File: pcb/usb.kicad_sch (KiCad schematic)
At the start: 16 parts, among them J601 USB_AB_Micro, J602 USB_B_Micro, J604 USB_B_Micro, U601 USBLC6-2P6, U602 CP2102N-Axx-xQFN20, U605 USBLC6-2P6

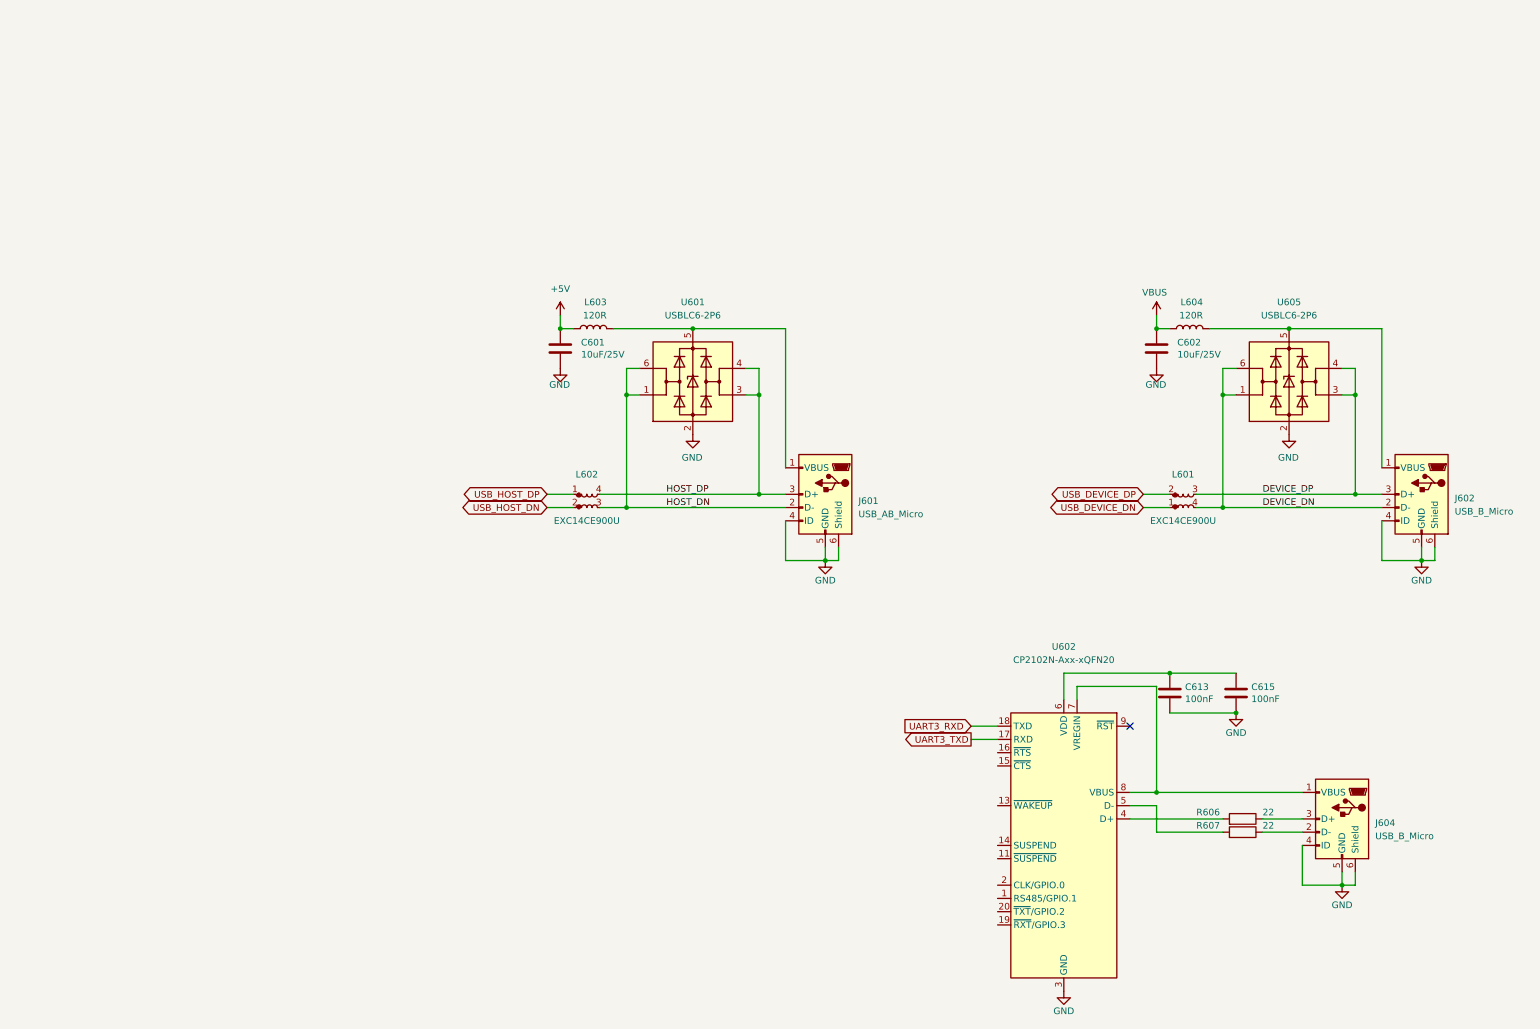
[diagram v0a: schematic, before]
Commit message: pcb: getting ready for r0.2 production
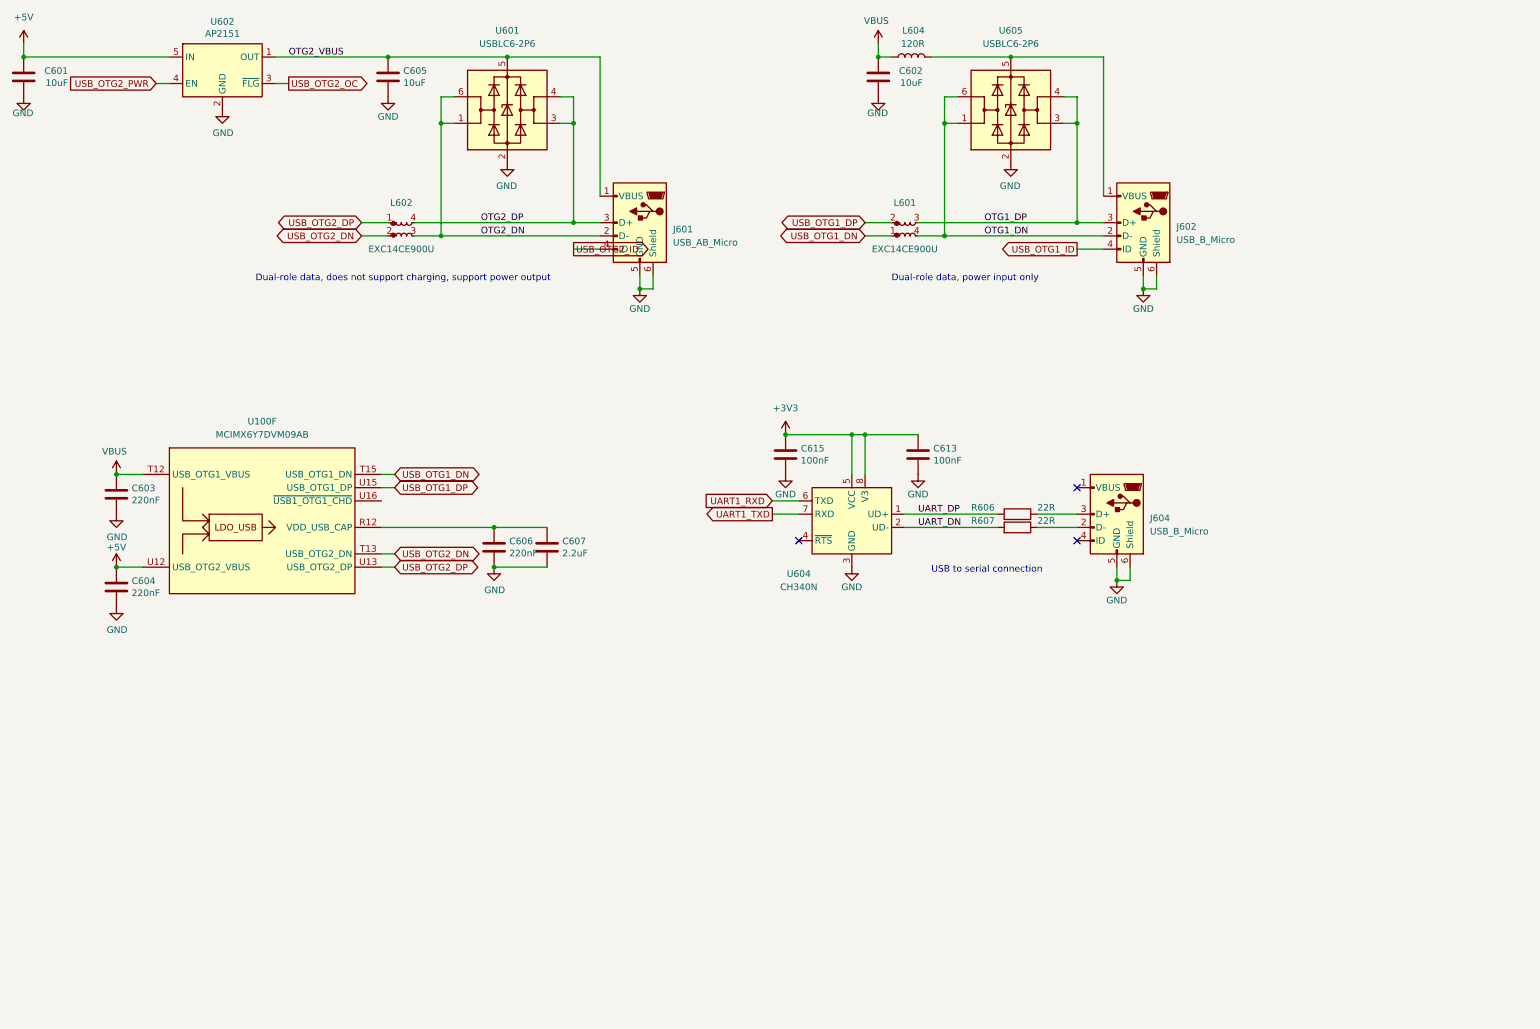
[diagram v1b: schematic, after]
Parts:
- removed L603: 120R, Inductor_SMD:L_0603_1608Metric, symbol Device:L
- removed U602: CP2102N-Axx-xQFN20, Package_DFN_QFN:SiliconLabs_QFN-20-1EP_3x3mm_P0.5mm_EP1.8x1.8mm, symbol Interface_USB:CP2102N-Axx-xQFN20
- added C603, C604, C606: 220nF, Capacitor_SMD:C_0402_1005Metric, symbol Device:C
- added C605: 10uF, Capacitor_SMD:C_0603_1608Metric, symbol Device:C
- added C607: 2.2uF, Capacitor_SMD:C_0402_1005Metric, symbol Device:C
- added U100: MCIMX6Y7DVM09AB, footprints:BGA-289_17x17_14.0x14.0mm, symbol symbols:MCIMX6Y7DVM09AB
- added U602: AP2151, Package_TO_SOT_SMD:SOT-23-5, symbol Power_Management:AP2171W
- added U604: CH340N, Package_SO:SO-8_3.9x4.9mm_P1.27mm, symbol symbols:CH340N
- C601, C602: value 10uF/25V -> 10uF; footprint Capacitor_SMD:C_0805_2012Metric -> Capacitor_SMD:C_0603_1608Metric
- R606, R607: value 22 -> 22R
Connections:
- net +5V: now also C604.1, U100.U12 (USB_OTG2_VBUS), U602.5 (IN)
- net GND: now also C603.2, C604.2, C605.2, C606.2, C607.2, U602.2 (GND), U604.3 (GND); no longer J601.4 (ID), J602.4 (ID), J604.4 (ID)
- net VBUS: now also C603.1, U100.T12 (USB_OTG1_VBUS)
- net OTG2_VBUS: now reaches J601.1 (VBUS), U601.5 (VBUS)
- net OTG2_VBUS: now also C605.1, U602.1 (OUT)
- net +3V3: now reaches C613.1, C615.1
- net +3V3: now also U604.5 (VCC), U604.8 (V3)
- net UART_DN: now reaches R607.2
- net UART_DN: now also U604.2 (UD-)
- net UART_DP: now reaches R606.2
- net UART_DP: now also U604.1 (UD+)
- net DEVICE_DN renamed OTG1_DN
- net DEVICE_DP renamed OTG1_DP
- net HOST_DN renamed OTG2_DN
- net HOST_DP renamed OTG2_DP
- net USB_DEVICE_DN renamed USB_OTG1_DN
- net USB_OTG1_DN: now also U100.T15 (USB_OTG1_DN)
- net USB_DEVICE_DP renamed USB_OTG1_DP
- net USB_OTG1_DP: now also U100.U15 (USB_OTG1_DP)
- net USB_HOST_DN renamed USB_OTG2_DN
- net USB_OTG2_DN: now also U100.T13 (USB_OTG2_DN)
- net USB_HOST_DP renamed USB_OTG2_DP
- net USB_OTG2_DP: now also U100.U13 (USB_OTG2_DP)
- new net: C606.1, C607.1, U100.R12 (VDD_USB_CAP)
- new net UART1_RXD: U604.6 (TXD)
- new net UART1_TXD: U604.7 (RXD)
- new net USB_OTG1_ID: J602.4 (ID)
- new net USB_OTG2_ID: J601.4 (ID)
- new net USB_OTG2_OC: U602.3 (~{FLG})
- new net USB_OTG2_PWR: U602.4 (EN)
- no-connect marks 1 -> 3
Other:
- note added: "Dual-role data, does not support charging, support power output"
- note added: "Dual-role data, power input only"
- note added: "USB to serial connection"
- moved on the sheet: C601, C602, C613, C615, J601, J602, J604, L601, L602, L604, R606, R607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
